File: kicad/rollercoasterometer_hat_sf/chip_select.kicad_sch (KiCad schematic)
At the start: 1 part, among them U1401 74LS138

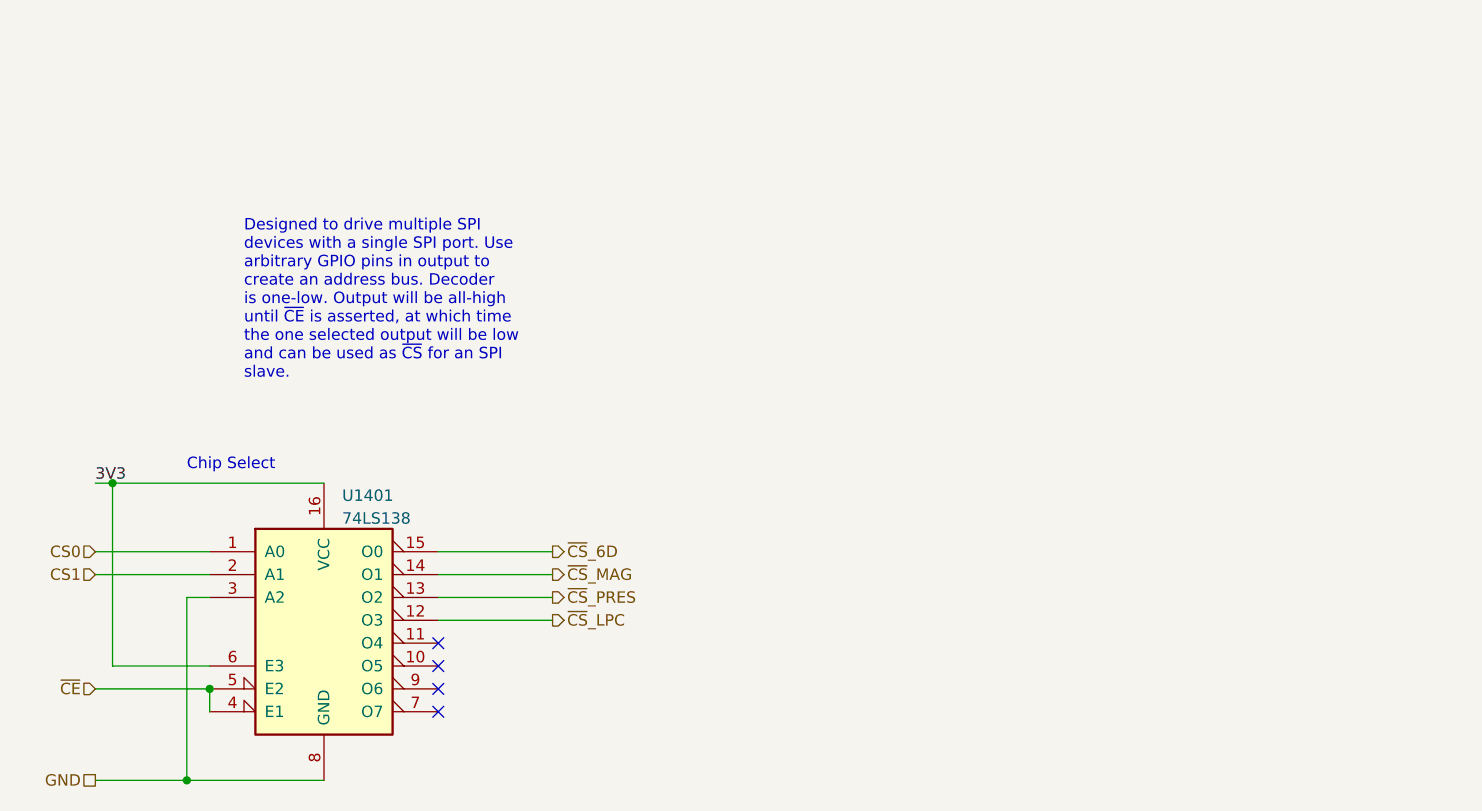
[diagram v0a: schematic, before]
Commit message: Commit as-ordered shipometer 23.03
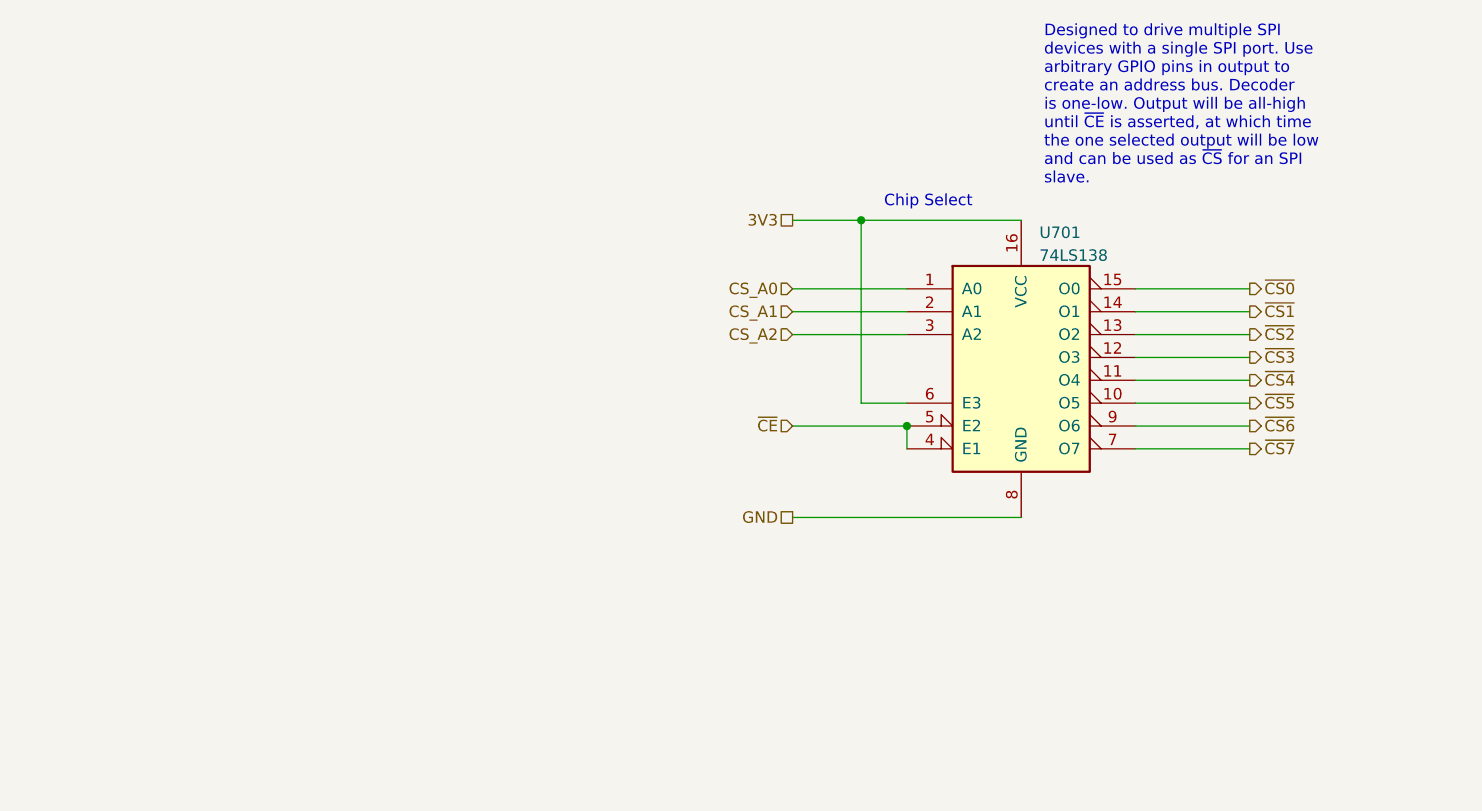
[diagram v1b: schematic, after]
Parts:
- removed U1401: 74LS138, Package_SO:TSSOP-16_4.4x5mm_P0.65mm, symbol 74xx:74LS138
- added U701: 74LS138, Package_SO:TSSOP-16_4.4x5mm_P0.65mm, symbol 74xx:74LS138
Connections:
- net 3V3: now also U701.16 (VCC), U701.6 (E3)
- net GND: now also U701.8 (GND)
- net ~{CE}: now also U701.4 (E1), U701.5 (E2)
- new net CS_A0: U701.1 (A0)
- new net CS_A1: U701.2 (A1)
- new net CS_A2: U701.3 (A2)
- new net ~{CS0}: U701.15 (O0)
- new net ~{CS1}: U701.14 (O1)
- new net ~{CS2}: U701.13 (O2)
- new net ~{CS3}: U701.12 (O3)
- new net ~{CS4}: U701.11 (O4)
- new net ~{CS5}: U701.10 (O5)
- new net ~{CS6}: U701.9 (O6)
- new net ~{CS7}: U701.7 (O7)
- no-connect marks 4 -> 0
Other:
- company: Kwan Systems -> (none)
- title: Rollercoasterometer -> (none)
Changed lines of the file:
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@@
 (kicad_sch (version 20211123) (generator eeschema)
-  (paper "USLetter")
-  (title_block
-    (title "Rollercoasterometer")
-    (date "2022-10-07")
-    (company "Kwan Systems")
+  (paper "A4")
+  (junction (at 110.49 74.93) (diameter 0) (color 0 0 0 0)
   )
-  (junction (at 27.305 104.14) (diameter 0) (color 0 0 0 0)
+  (junction (at 115.57 97.79) (diameter 0) (color 0 0 0 0)
   )
-  (junction (at 35.56 137.16) (diameter 0) (color 0 0 0 0)
-  )
-  (junction (at 38.1 127) (diameter 0) (color 0 0 0 0)
-  )
-  (no_connect (at 63.5 129.54))
-  (no_connect (at 63.5 127))
-  (no_connect (at 63.5 124.46))
-  (no_connect (at 63.5 121.92))
-  (wire (pts (xy 25.4 114.3) (xy 38.1 114.3))
+  (wire (pts (xy 102.87 85.09) (xy 115.57 85.09))
     (stroke (width 0) (type default) (color 0 0 0 0))
   )
-  (wire (pts (xy 63.5 111.76) (xy 76.2 111.76))
+  (wire (pts (xy 140.97 92.71) (xy 153.67 92.71))
     (stroke (width 0) (type default) (color 0 0 0 0))
   )
-  (wire (pts (xy 63.5 116.84) (xy 76.2 116.84))
+  (wire (pts (xy 140.97 90.17) (xy 153.67 90.17))
     (stroke (width 0) (type default) (color 0 0 0 0))
   )
-  (wire (pts (xy 63.5 114.3) (xy 76.2 114.3))
+  (wire (pts (xy 140.97 87.63) (xy 153.67 87.63))
     (stroke (width 0) (type default) (color 0 0 0 0))
   )
-  (wire (pts (xy 25.4 127) (xy 38.1 127))
+  (wire (pts (xy 115.57 97.79) (xy 115.57 100.33))
     (stroke (width 0) (type default) (color 0 0 0 0))
   )
-  (wire (pts (xy 35.56 137.16) (xy 50.8 137.16))
+  (wire (pts (xy 102.87 107.95) (xy 128.27 107.95))
     (stroke (width 0) (type default) (color 0 0 0 0))
   )
-  (wire (pts (xy 25.4 111.76) (xy 38.1 111.76))
+  (wire (pts (xy 140.97 82.55) (xy 153.67 82.55))
     (stroke (width 0) (type default) (color 0 0 0 0))
   )
-  (wire (pts (xy 25.4 104.14) (xy 27.305 104.14))
+  (wire (pts (xy 102.87 87.63) (xy 115.57 87.63))
     (stroke (width 0) (type default) (color 0 0 0 0))
   )
-  (wire (pts (xy 35.56 116.84) (xy 38.1 116.84))
+  (wire (pts (xy 140.97 95.25) (xy 153.67 95.25))
     (stroke (width 0) (type default) (color 0 0 0 0))
   )
-  (wire (pts (xy 27.305 104.14) (xy 27.305 124.46))
+  (wire (pts (xy 102.87 74.93) (xy 110.49 74.93))
     (stroke (width 0) (type default) (color 0 0 0 0))
   )
-  (wire (pts (xy 27.305 104.14) (xy 50.8 104.14))
+  (wire (pts (xy 140.97 97.79) (xy 153.67 97.79))
     (stroke (width 0) (type default) (color 0 0 0 0))
   )
-  (wire (pts (xy 63.5 119.38) (xy 76.2 119.38))
+  (wire (pts (xy 110.49 74.93) (xy 128.27 74.93))
     (stroke (width 0) (type default) (color 0 0 0 0))
   )
-  (wire (pts (xy 35.56 116.84) (xy 35.56 137.16))
+  (wire (pts (xy 110.49 74.93) (xy 110.49 95.25))
     (stroke (width 0) (type default) (color 0 0 0 0))
   )
-  (wire (pts (xy 27.305 124.46) (xy 38.1 124.46))
+  (wire (pts (xy 110.49 95.25) (xy 115.57 95.25))
     (stroke (width 0) (type default) (color 0 0 0 0))
   )
-  (wire (pts (xy 38.1 127) (xy 38.1 129.54))
+  (wire (pts (xy 140.97 85.09) (xy 153.67 85.09))
     (stroke (width 0) (type default) (color 0 0 0 0))
   )
-  (wire (pts (xy 25.4 137.16) (xy 35.56 137.16))
+  (wire (pts (xy 102.87 82.55) (xy 115.57 82.55))
     (stroke (width 0) (type default) (color 0 0 0 0))
   )
-  (text "Designed to drive multiple SPI\ndevices with a single SPI port. Use\narbitrary GPIO pins in output to\ncreate an address bus. Decoder\nis one-low. Output will be all-high\nuntil ~{CE} is asserted, at which time\nthe one selected output will be low\nand can be used as ~{CS} for an SPI\nslave."
-    (at 41.91 92.71 0)
+  (wire (pts (xy 102.87 97.79) (xy 115.57 97.79))
+    (stroke (width 0) (type default) (color 0 0 0 0))
+  )
+  (wire (pts (xy 140.97 100.33) (xy 153.67 100.33))
+    (stroke (width 0) (type default) (color 0 0 0 0))
+  )
+  (text "Chip Select" (at 113.03 73.66 0)
     (effects (font (size 1.27 1.27)) (justify left bottom))
   )
-  (text "Chip Select" (at 35.56 102.87 0)
+  (text "Designed to drive multiple SPI\ndevices with a single SPI port. Use\narbitrary GPIO pins in output to\ncreate an address bus. Decoder\nis one-low. Output will be all-high\nuntil ~{CE} is asserted, at which time\nthe one selected output will be low\nand can be used as ~{CS} for an SPI\nslave."
+    (at 130.81 71.12 0)
     (effects (font (size 1.27 1.27)) (justify left bottom))
   )
-  (label "3V3" (at 25.4 104.14 0)
-    (effects (font (size 1.27 1.27)) (justify left bottom))
+  (hierarchical_label "~{CS7}" (shape output) (at 153.67 100.33 0)
+    (effects (font (size 1.27 1.27)) (justify left))
   )
-  (hierarchical_label "~{CE}" (shape input) (at 25.4 127 180)
+  (hierarchical_label "~{CS4}" (shape output) (at 153.67 92.71 0)
+    (effects (font (size 1.27 1.27)) (justify left))
+  )
+  (hierarchical_label "CS_A0" (shape input) (at 102.87 82.55 180)
     (effects (font (size 1.27 1.27)) (justify right))
   )
-  (hierarchical_label "GND" (shape passive) (at 25.4 137.16 180)
+  (hierarchical_label "~{CS3}" (shape output) (at 153.67 90.17 0)
+    (effects (font (size 1.27 1.27)) (justify left))
+  )
+  (hierarchical_label "GND" (shape passive) (at 102.87 107.95 180)
     (effects (font (size 1.27 1.27)) (justify right))
   )
-  (hierarchical_label "~{CS}_LPC" (shape output) (at 76.2 119.38 0)
+  (hierarchical_label "~{CS2}" (shape output) (at 153.67 87.63 0)
     (effects (font (size 1.27 1.27)) (justify left))
   )
-  (hierarchical_label "CS0" (shape input) (at 25.4 111.76 180)
+  (hierarchical_label "CS_A2" (shape input) (at 102.87 87.63 180)
     (effects (font (size 1.27 1.27)) (justify right))
   )
-  (hierarchical_label "~{CS}_6D" (shape output) (at 76.2 111.76 0)
+  (hierarchical_label "~{CS5}" (shape output) (at 153.67 95.25 0)
     (effects (font (size 1.27 1.27)) (justify left))
   )
-  (hierarchical_label "~{CS}_PRES" (shape output) (at 76.2 116.84 0)
+  (hierarchical_label "~{CS0}" (shape output) (at 153.67 82.55 0)
     (effects (font (size 1.27 1.27)) (justify left))
   )
-  (hierarchical_label "~{CS}_MAG" (shape output) (at 76.2 114.3 0)
+  (hierarchical_label "3V3" (shape passive) (at 102.87 74.93 180)
+    (effects (font (size 1.27 1.27)) (justify right))
+  )
+  (hierarchical_label "CS_A1" (shape input) (at 102.87 85.09 180)
+    (effects (font (size 1.27 1.27)) (justify right))
+  )
+  (hierarchical_label "~{CS6}" (shape output) (at 153.67 97.79 0)
     (effects (font (size 1.27 1.27)) (justify left))
   )
-  (hierarchical_label "CS1" (shape input) (at 25.4 114.3 180)
+  (hierarchical_label "~{CS1}" (shape output) (at 153.67 85.09 0)
+    (effects (font (size 1.27 1.27)) (justify left))
+  )
+  (hierarchical_label "~{CE}" (shape input) (at 102.87 97.79 180)
     (effects (font (size 1.27 1.27)) (justify right))
   )
-  (symbol (lib_id "74xx:74LS138") (at 50.8 119.38 0) (unit 1)
+  (symbol (lib_id "74xx:74LS138") (at 128.27 90.17 0) (unit 1)
     (in_bom yes) (on_board yes) (fields_autoplaced)
-    (property "Reference" "U1401" (id 0) (at 52.8194 105.5202 0)
+    (property "Reference" "U701" (id 0) (at 130.2894 76.3102 0)
       (effects (font (size 1.27 1.27)) (justify left))
     )
-    (property "Value" "74LS138" (id 1) (at 52.8194 108.0571 0)
+    (property "Value" "74LS138" (id 1) (at 130.2894 78.8471 0)
       (effects (font (size 1.27 1.27)) (justify left))
     )
-    (property "Footprint" "Package_SO:TSSOP-16_4.4x5mm_P0.65mm" (id 2) (at 50.8 119.38 0)
+    (property "Footprint" "Package_SO:TSSOP-16_4.4x5mm_P0.65mm" (id 2) (at 128.27 90.17 0)
       (effects (font (size 1.27 1.27)) hide)
     )
-    (property "Datasheet" "http://www.ti.com/lit/gpn/sn74LS138" (id 3) (at 50.8 119.38 0)
+    (property "Datasheet" "http://www.ti.com/lit/gpn/sn74LS138" (id 3) (at 128.27 90.17 0)
       (effects (font (size 1.27 1.27)) hide)
     )
-    (property "Mouser" "771-74LVC138APW-T" (id 4) (at 50.8 119.38 0)
+    (property "Mouser" "771-74LVC138APW-T" (id 4) (at 128.27 90.17 0)
       (effects (font (size 1.27 1.27)) hide)
     )
-    (property "Purpose" "SPI Chip Select Decoder" (id 5) (at 50.8 119.38 0)
+    (property "Purpose" "SPI Chip Select Decoder" (id 5) (at 128.27 90.17 0)
       (effects (font (size 1.27 1.27)) hide)
     )
